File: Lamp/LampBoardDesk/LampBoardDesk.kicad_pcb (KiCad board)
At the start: 2 copper layers, 119.1 x 80.7 mm, 87 parts, among them IC1 L7805ABD2T-TR, IC2 SN74LVC2T45DCUR, J1 DS1023-1x3SF11, J2 DS1023-1x3SF11, J3 284514-3, J4 DC-005-A250, Q1 CMN3406M, SW1 PEC11R, SW2 MT-0-102, U1 RP2040, U2 W25Q128JVS, U3 LTV357T-B, U4 LTV357T-B, Y1 ABM8-272-T3

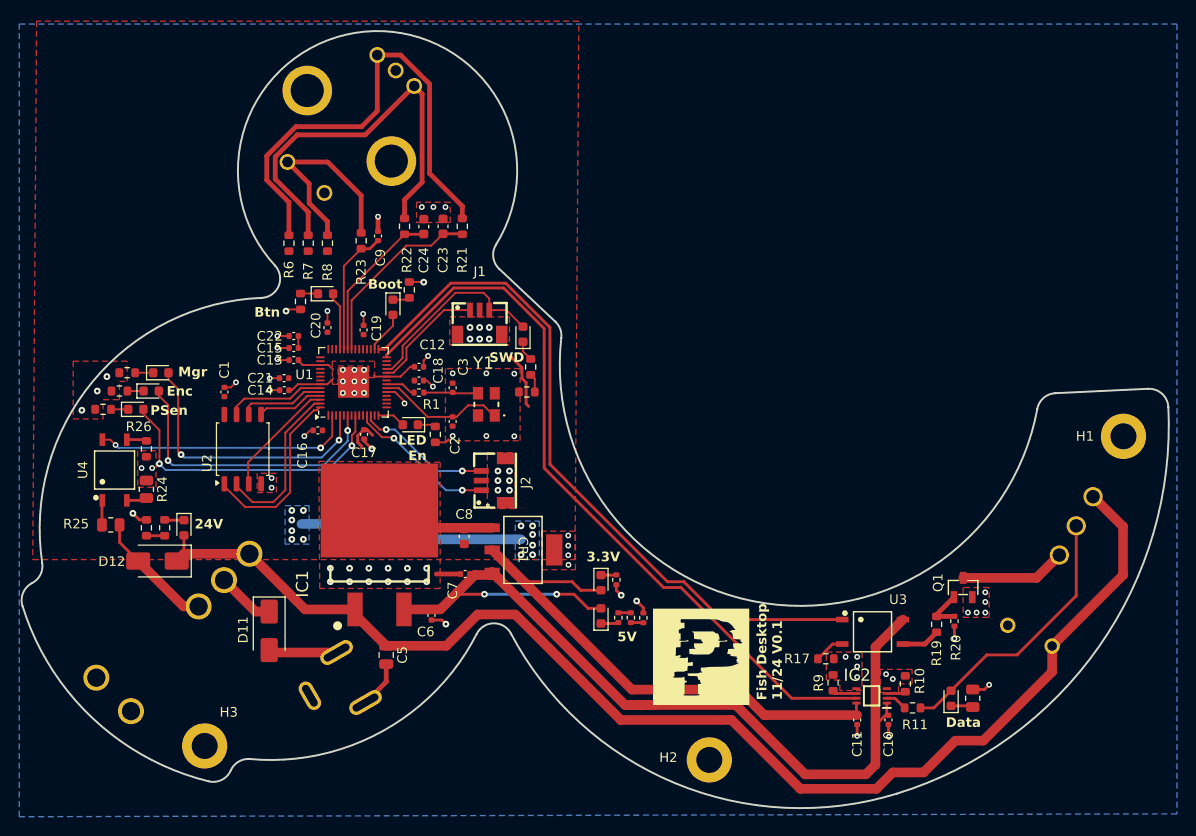
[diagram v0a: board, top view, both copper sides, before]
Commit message: Final version ready to roll
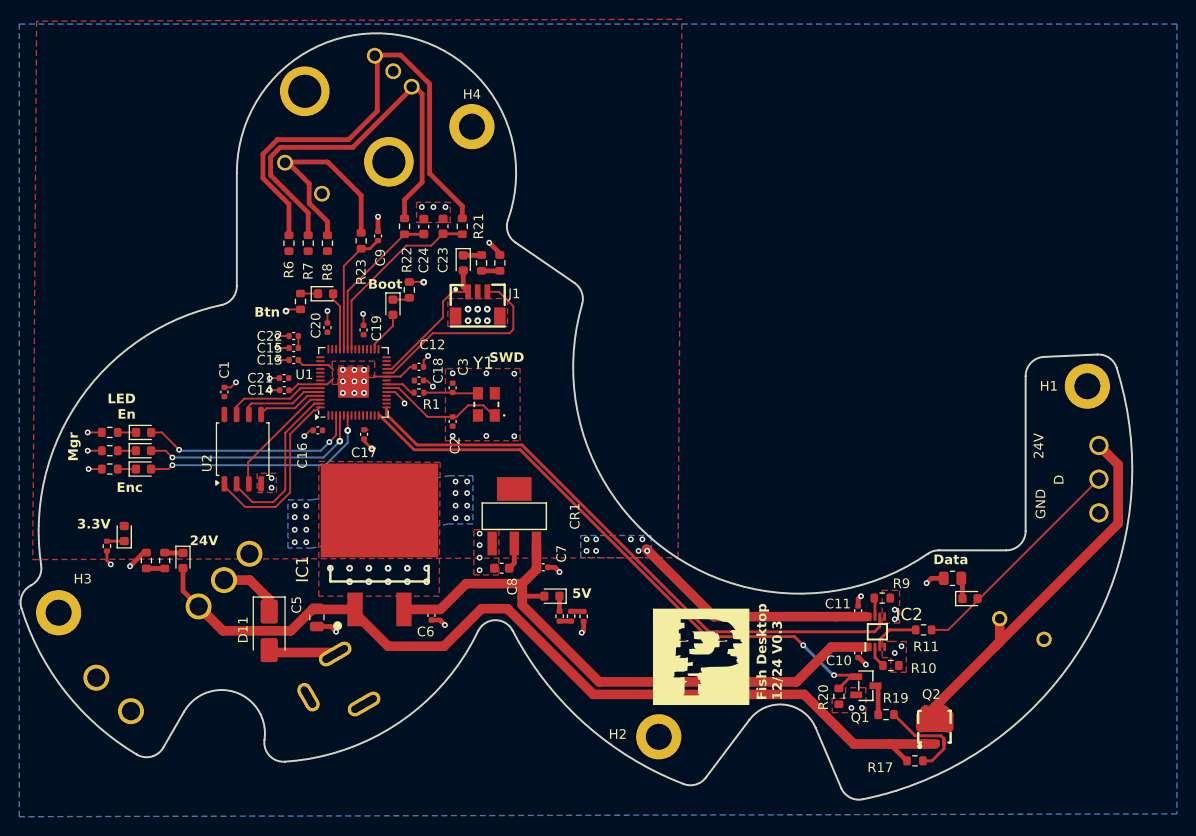
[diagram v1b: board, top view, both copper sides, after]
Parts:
- removed D12: D_Schottky, Diode_SMD:D_SMA
- removed D13: GREEN, LED_SMD:LED_0603_1608Metric
- removed J2: DS1023-1x3SF11, easyeda2kicad:CONN-SMD-3P-P1.00_BM03B-SRSS-TB-LF-SN
- removed R24, R25: 2.4k, Resistor_SMD:R_0805_2012Metric
- removed R26, R27: 330, Resistor_SMD:R_0603_1608Metric
- removed U3, U4: LTV357T-B, easyeda2kicad:SOP-4_L4.4-W4.0-P2.54-LS7.0-TL
- added H4: MountingHole_Pad, MountingHole:MountingHole_2.7mm_M2.5_DIN965_Pad, F.Cu at (59.0, 22.6)
- added Q2: FH38P03G6, easyeda2kicad:DFN-8_L3.3-W3.3-P0.65-BL-EP, F.Cu at (107.0, 85.0)
- CR1: footprint LD1117S33CTR:SOT-223_STM -> easyeda2kicad:SOT-223-4_L6.5-W3.5-P2.30-LS7.0-BR
- R17: value 330 -> 10k
- R19: value 100 -> 10k
- R20: value 1K -> 10k; footprint Resistor_SMD:R_0402_1005Metric -> Resistor_SMD:R_0603_1608Metric
- R21, R22, R23, R8: value 10K -> 10k
- moved R4 53.0 mm to (21.1, 66.2)
- moved D3 49.8 mm to (22.9, 64.9), turned to 90 degrees
- moved R18 33.8 mm to (21.4, 54.4), turned to 180 degrees
- moved D10 27.7 mm to (24.9, 54.4), turned to 0 degrees
- moved H3 20.5 mm to (16.1, 73.1)
- moved Q1 14.4 mm to (99.9, 80.7), turned to 180 degrees
- moved R20 14.3 mm to (97.1, 81.8), turned to 90 degrees
- moved R17 14.1 mm to (105.0, 88.5), turned to 180 degrees
- moved R28 13.7 mm to (61.9, 36.8), turned to -90 degrees
- moved R15 12.6 mm to (108.9, 69.5), turned to 180 degrees
- moved R5 11.9 mm to (60.0, 36.8)
- moved C11 11.4 mm to (99.1, 72.9), turned to 90 degrees
- moved R19 10.7 mm to (102.0, 83.7), turned to 0 degrees
- moved D8 10.5 mm to (110.7, 71.7), turned to 0 degrees
- moved R9 10.2 mm to (101.6, 71.6), turned to 0 degrees
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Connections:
- C4 pad 1: +24V -> Net-(C4-Pad1)
- C7 pad 1: +5V -> GND
- C7 pad 2: GND -> +5V
- C8 pad 1: +3.3V -> GND
- C8 pad 2: GND -> +3.3V
- IC2 pad 6: Net-(IC2-B2) -> /LED_D
- IC2 pad 7: /LED_D -> Net-(IC2-B1)
- J1 pad 1: /SW_CLK -> /SW_D
- J1 pad 3: /SW_D -> /SW_CLK
- J3 pad 1: Net-(Q1-D) -> GND
- J3 pad 3: +24V -> Net-(C4-Pad1)
- Q1 pad 1: Net-(Q1-G) -> /LED_EN
- R10 pad 1: GND -> Net-(IC2-A1)
- R10 pad 2: Net-(IC2-A2) -> GND
- R11 pad 2: Net-(IC2-A1) -> Net-(IC2-A2)
- R17 pad 1: Net-(R17-Pad1) -> Net-(Q2-G)
- R17 pad 2: GND -> +24V
- R19 pad 1: Net-(Q1-G) -> Net-(Q1-D)
- R19 pad 2: Net-(R19-Pad2) -> Net-(Q2-G)
- R20 pad 1: Net-(Q1-G) -> GND
- R20 pad 2: GND -> /LED_EN
- R9 pad 1: GND -> Net-(IC2-B1)
- R9 pad 2: Net-(IC2-B2) -> GND
- SW2 pad 1: +24V -> unconnected-(SW2-Pad1)
- SW2 pad 3: /P_SEN -> +24V
- U1 pad 11: /UART_TX -> unconnected-(U1-GPIO8-Pad11)
- U1 pad 12: /UART_RX -> unconnected-(U1-GPIO9-Pad12)
- U1 pad 14: /LED_EN_LED -> /LED_EN
- U1 pad 15: unconnected-(U1-GPIO12-Pad15) -> /LED_D
- U1 pad 2: /P_SEN_O -> unconnected-(U1-GPIO0-Pad2)
- U1 pad 28: /LED_D -> unconnected-(U1-GPIO17-Pad28)
- U1 pad 29: /LED_EN -> unconnected-(U1-GPIO18-Pad29)
- U1 pad 3: unconnected-(U1-GPIO1-Pad3) -> /LED_EN_LED
- U1 pad 8: /P_SEN_LED -> unconnected-(U1-GPIO6-Pad8)
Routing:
- net +3.3V: track 88.9 -> 31.1 mm, vias 12 -> 24
- net Net-(C4-Pad1): track 0.00 -> 46.5 mm
- net +24V: track 134.8 -> 95.4 mm
- net +5V: track 98.3 -> 63.3 mm, vias 2 -> 0
- net /P_SEN_LED: track 30.9 -> 0.00 mm, vias 2 -> 0
- net /P_SEN_O: track 26.9 -> 0.00 mm, vias 2 -> 0
- net /LED_EN_LED: track 2.91 -> 22.7 mm, vias 0 -> 2
- net /LED_D: track 78.0 -> 62.5 mm
- net /UART_TX: track 15.5 -> 0.00 mm, vias 2 -> 0
- net /UART_RX: track 14.2 -> 0.00 mm, vias 2 -> 0
- net /P_SEN: track 12.8 -> 0.00 mm
- net /LED_EN: track 73.9 -> 63.1 mm, vias 0 -> 2
- net GND: track 54.0 -> 43.8 mm, vias 88 -> 76
- net Net-(Q2-G): track 0.00 -> 9.98 mm
- net /SW_CLK: track 12.1 -> 20.7 mm
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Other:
- board size 119.1 x 80.7 mm -> 115.4 x 79.6 mm
- board text added: "Fish Desktop 12/24 V0.3"
- board text removed: "Fish Desktop 11/24 V0.1"
- board text removed: "PSen"
